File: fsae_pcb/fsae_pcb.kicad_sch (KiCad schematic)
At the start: 0 parts

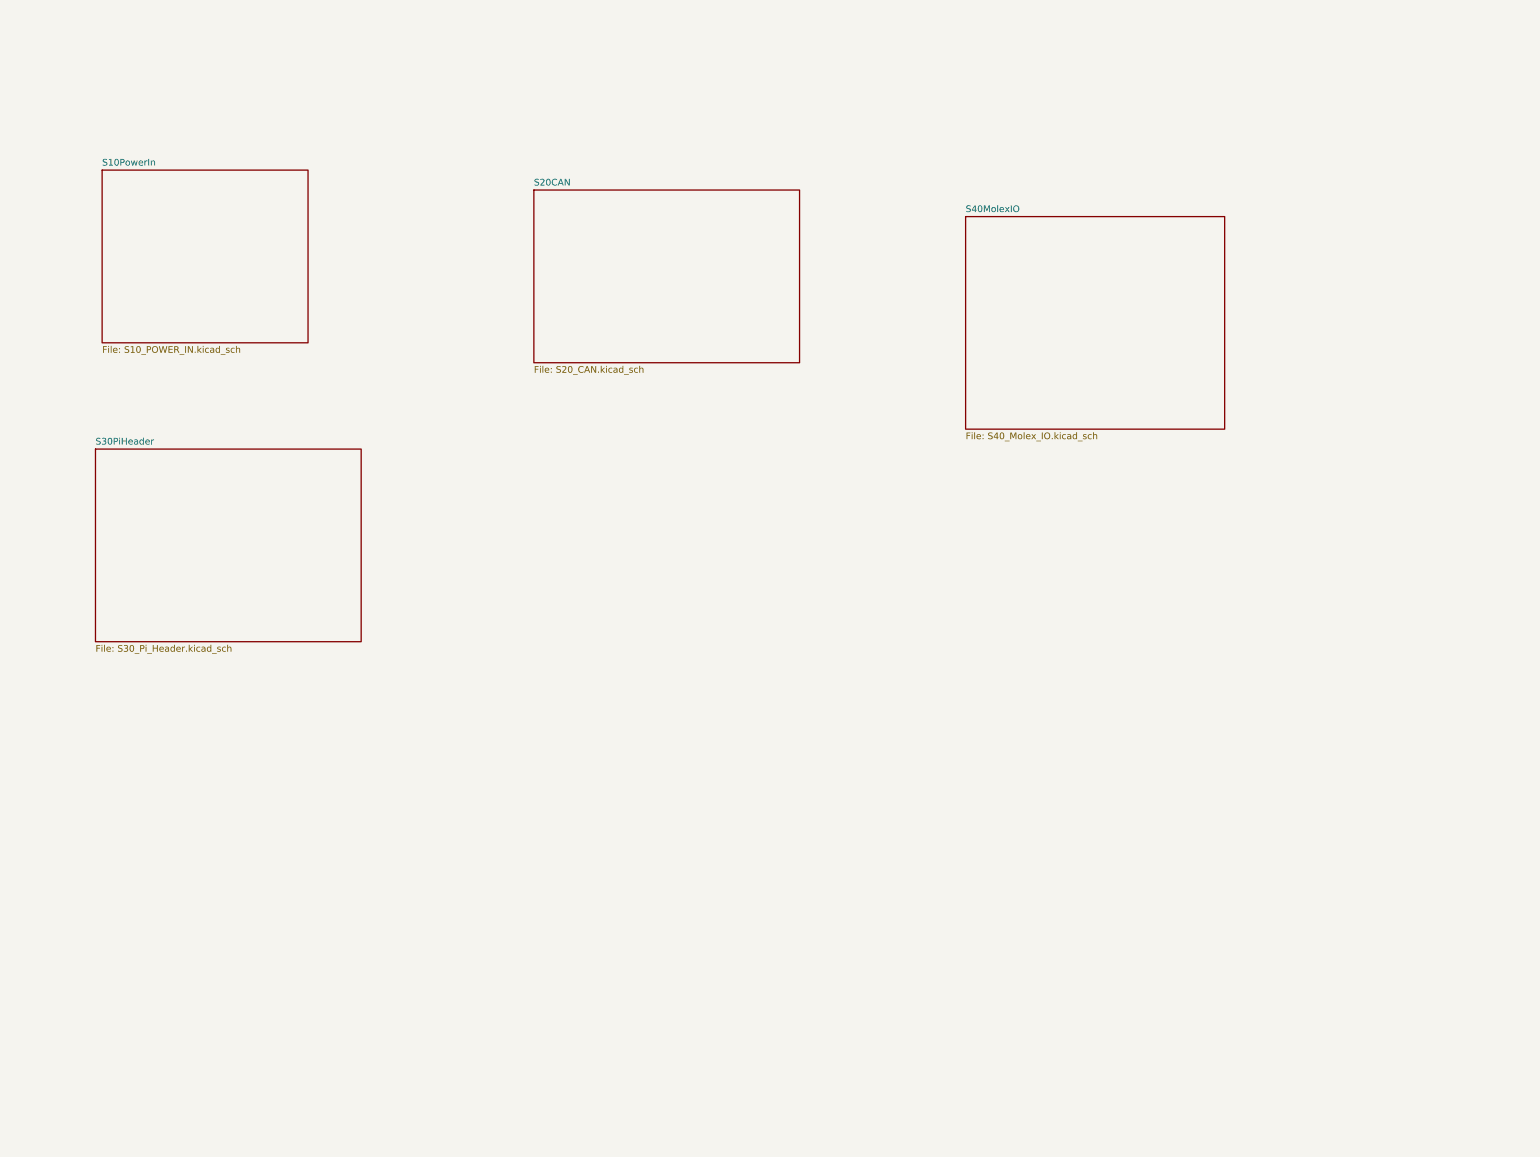
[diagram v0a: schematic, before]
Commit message: new main pcb design
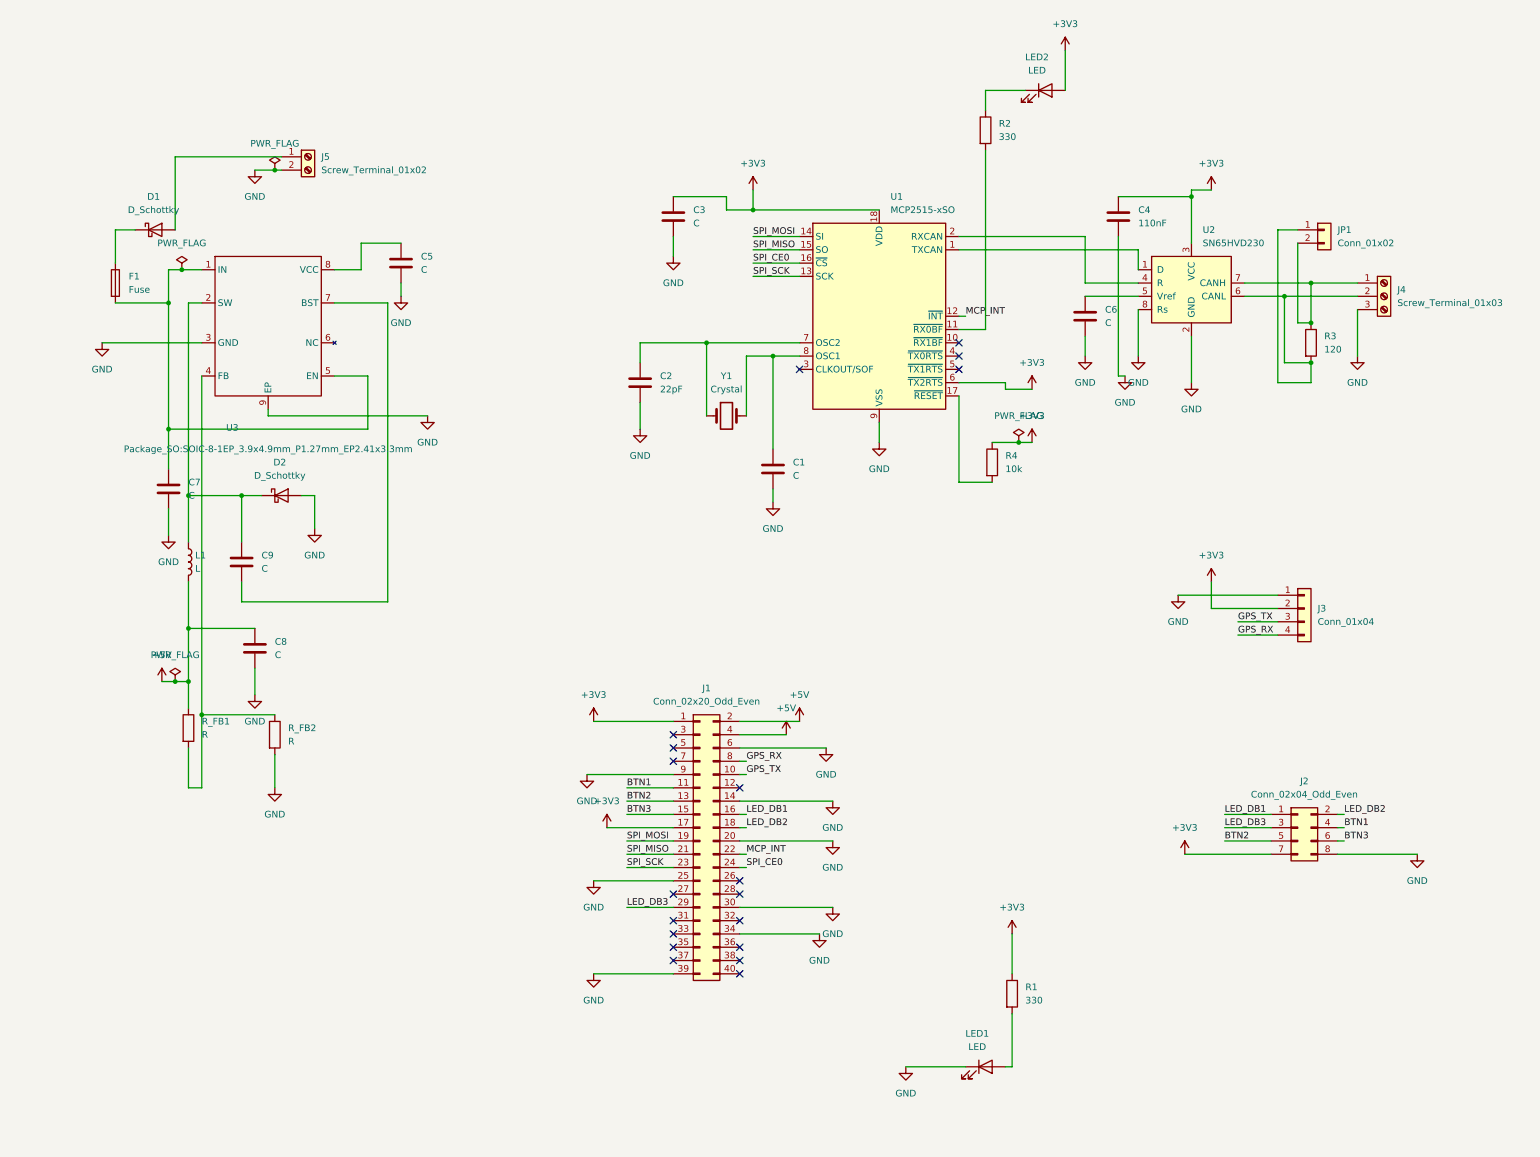
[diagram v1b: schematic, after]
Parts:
- added C1, C3, C5, C6, C7, C8, C9: C, symbol Device:C
- added C2: 22pF, symbol Device:C
- added C4: 110nF, symbol Device:C
- added D1, D2: D_Schottky, symbol Device:D_Schottky
- added F1: Fuse, symbol Device:Fuse
- added J1: Conn_02x20_Odd_Even, symbol Connector_Generic:Conn_02x20_Odd_Even
- added J2: Conn_02x04_Odd_Even, symbol Connector_Generic:Conn_02x04_Odd_Even
- added J3: Conn_01x04, symbol Connector_Generic:Conn_01x04
- added J4: Screw_Terminal_01x03, symbol Connector:Screw_Terminal_01x03
- added J5: Screw_Terminal_01x02, symbol Connector:Screw_Terminal_01x02
- added JP1: Conn_01x02, symbol Connector_Generic:Conn_01x02
- added L1: L, symbol Device:L
- added LED1, LED2: LED, symbol Device:LED
- added R1, R2: 330, symbol Device:R
- added R3: 120, symbol Device:R
- added R4: 10k, symbol Device:R
- added R_FB1, R_FB2: R, symbol Device:R
- added U1: MCP2515-xSO, Package_SO:SOIC-18W_7.5x11.6mm_P1.27mm, symbol Interface_CAN_LIN:MCP2515-xSO
- added U2: SN65HVD230, Package_SO:SOIC-8_3.9x4.9mm_P1.27mm, symbol Interface_CAN_LIN:SN65HVD230
- added U3: ~, Package_SO:SOIC-8-1EP_3.9x4.9mm_P1.27mm_EP2.41x3.3mm, symbol MP1584EN:MP_1
- added Y1: Crystal, symbol Device:Crystal
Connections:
- new net: C9.1, D2.1 (K), L1.1, U3.2 (SW)
- new net: C9.2, U3.7 (BST)
- new net: J4.2 (Pin_2), JP1.1 (Pin_1), R3.2, U2.6 (CANL)
- new net: J4.1 (Pin_1), JP1.2 (Pin_2), R3.1, U2.7 (CANH)
- new net: C2.1, U1.7 (OSC2), Y1.1
- new net: C1.1, U1.8 (OSC1), Y1.2
- new net: R_FB1.2, R_FB2.1, U3.4 (FB)
- new net: C5.1, U3.8 (VCC)
- new net: D1.1 (K), F1.1
- new net: D1.2 (A), J5.1 (Pin_1)
- new net: LED1.2 (A), R1.2
- new net: LED2.1 (K), R2.1
- new net: R2.2, U1.11 (~{RX0BF})
- new net: U1.1 (TXCAN), U2.1 (D)
- new net: U1.2 (RXCAN), U2.4 (R)
- new net: C6.1, U2.5 (Vref)
- new net: C7.1, F1.2, U3.1 (IN), U3.5 (EN)
- new net: R4.2, U1.17 (~{RESET})
- new net +3V3: C3.1, C4.1, J1.1 (Pin_1), J1.17 (Pin_17), J2.7 (Pin_7), J3.2 (Pin_2), LED2.2 (A), R1.1, R4.1, U1.18 (VDD), U1.6 (~{TX2RTS}), U2.3 (VCC)
- new net +5V: C8.1, J1.2 (Pin_2), J1.4 (Pin_4), L1.2, R_FB1.1
- new net BTN1: J1.11 (Pin_11), J2.4 (Pin_4)
- new net BTN2: J1.13 (Pin_13), J2.5 (Pin_5)
- new net BTN3: J1.15 (Pin_15), J2.6 (Pin_6)
- new net GND: C1.2, C2.2, C3.2, C4.2, C5.2, C6.2, C7.2, C8.2, D2.2 (A), J1.14 (Pin_14), J1.20 (Pin_20), J1.25 (Pin_25), J1.30 (Pin_30), J1.34 (Pin_34), J1.39 (Pin_39), J1.6 (Pin_6), J1.9 (Pin_9), J2.8 (Pin_8), J3.1 (Pin_1), J4.3 (Pin_3), J5.2 (Pin_2), LED1.1 (K), R_FB2.2, U1.9 (VSS), U2.2 (GND), U2.8 (Rs), U3.3 (GND), U3.9 (EP)
- new net GPS_RX: J1.8 (Pin_8), J3.4 (Pin_4)
- new net GPS_TX: J1.10 (Pin_10), J3.3 (Pin_3)
- new net LED_DB1: J1.16 (Pin_16), J2.1 (Pin_1)
- new net LED_DB2: J1.18 (Pin_18), J2.2 (Pin_2)
- new net LED_DB3: J1.29 (Pin_29), J2.3 (Pin_3)
- new net MCP_INT: J1.22 (Pin_22), U1.12 (~{INT})
- new net SPI_CE0: J1.24 (Pin_24), U1.16 (~{CS})
- new net SPI_MISO: J1.21 (Pin_21), U1.15 (SO)
- new net SPI_MOSI: J1.19 (Pin_19), U1.14 (SI)
- new net SPI_SCK: J1.23 (Pin_23), U1.13 (SCK)
- no-connect marks 0 -> 19
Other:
- removed sheet S10PowerIn
- removed sheet S20CAN
- removed sheet S30PiHeader
- removed sheet S40MolexIO

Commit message: finished product
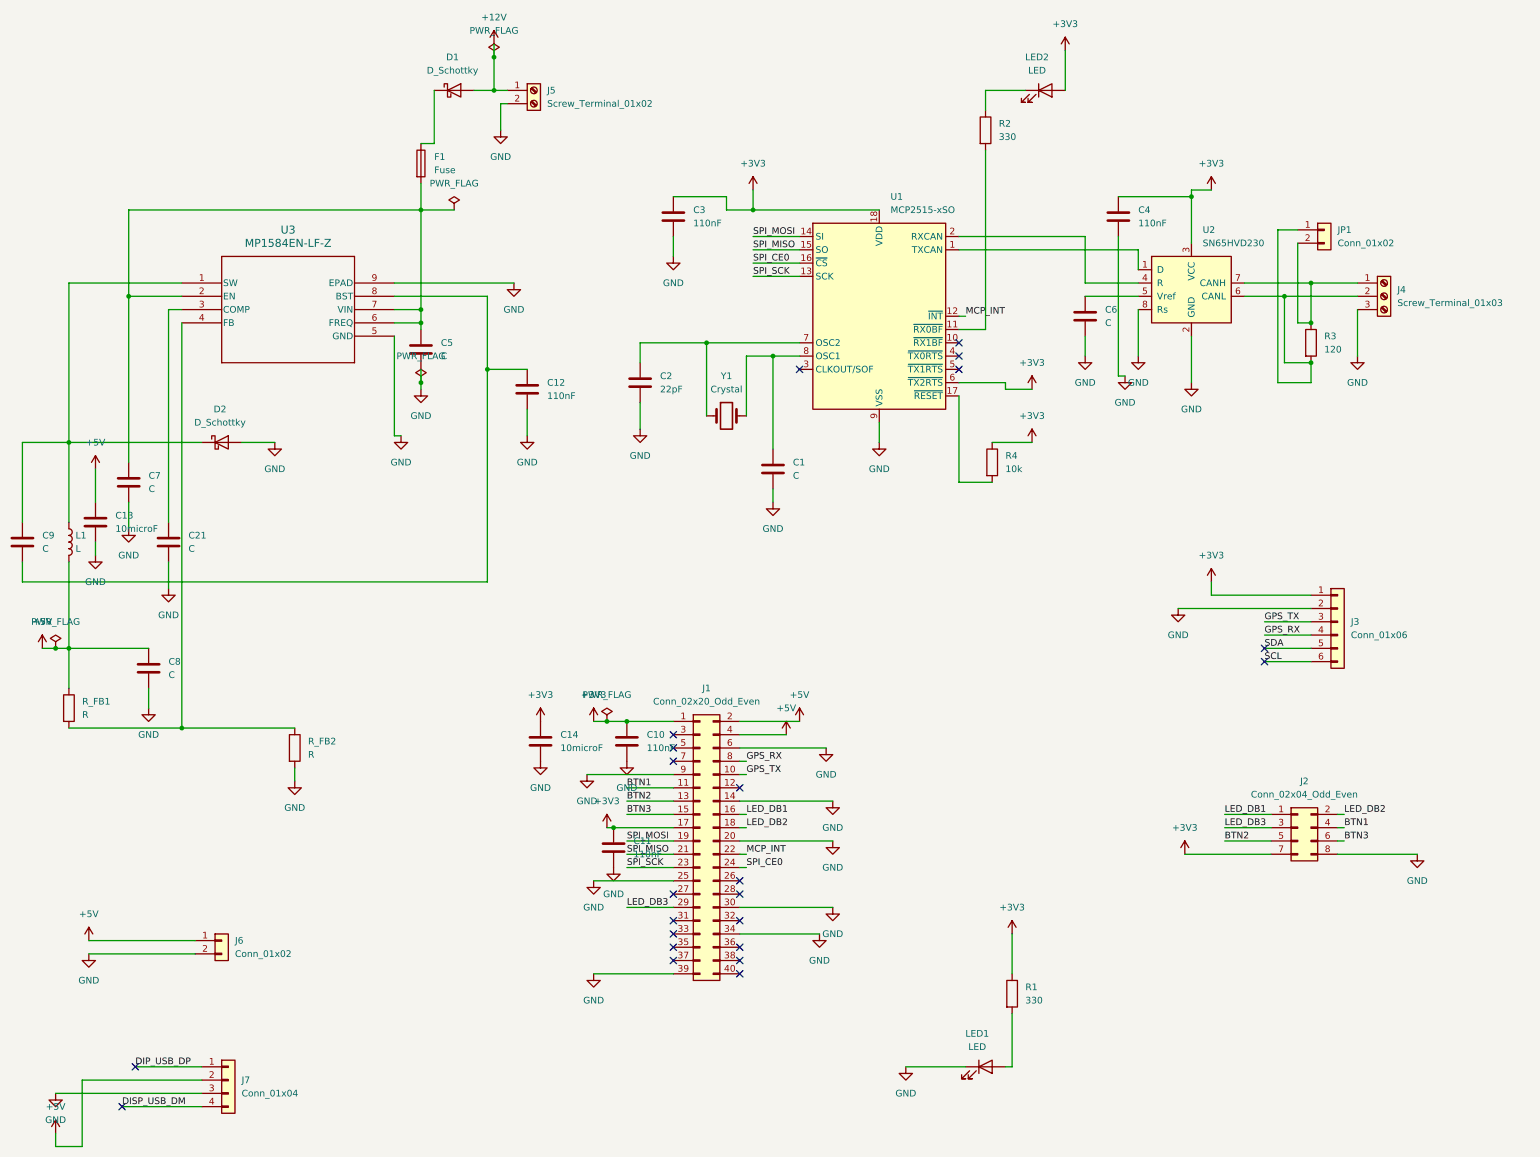
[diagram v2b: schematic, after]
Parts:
- removed J3: Conn_01x04, symbol Connector_Generic:Conn_01x04
- removed U3: ~, Package_SO:SOIC-8-1EP_3.9x4.9mm_P1.27mm_EP2.41x3.3mm, symbol MP1584EN:MP_1
- added C10, C11, C12: 110nF, Capacitor_SMD:C_0805_2012Metric, symbol Device:C
- added C13, C14: 10microF, Capacitor_SMD:C_0805_2012Metric, symbol Device:C
- added C21: C, Capacitor_SMD:C_0805_2012Metric, symbol Device:C
- added J3: Conn_01x06, Connector_PinHeader_2.54mm:PinHeader_1x06_P2.54mm_Vertical, symbol Connector_Generic:Conn_01x06
- added J6: Conn_01x02, Connector_PinHeader_2.54mm:PinHeader_1x02_P2.54mm_Vertical, symbol Connector_Generic:Conn_01x02
- added J7: Conn_01x04, Connector_PinHeader_2.54mm:PinHeader_1x04_P2.54mm_Vertical, symbol Connector_Generic:Conn_01x04
- added U3: MP1584EN-LF-Z, Package_SO:SOIC-8-1EP_3.9x4.9mm_P1.27mm_EP2.29x3mm, symbol 2026-03-05_05-11-51:MP1584EN-LF-Z
- C1, C2, C4, C5, C6, C9: footprint (none) -> Capacitor_SMD:C_0805_2012Metric
- C3: value C -> 110nF; footprint (none) -> Capacitor_SMD:C_0805_2012Metric
- C7, C8: footprint (none) -> Capacitor_SMD:C_1210_3225Metric
- D1, D2: footprint (none) -> Diode_SMD:D_SMA
- F1: footprint (none) -> Fuse:Fuseholder_Clip-5x20mm_Littelfuse_111_Inline_P20.00x5.00mm_D1.05mm_Horizontal
- J1: footprint (none) -> RPi_Hat.pretty-master:Pin_Header_Straight_2x20
- J2: footprint (none) -> Connector_Molex:Molex_Micro-Fit_3.0_43045-0812_2x04_P3.00mm_Vertical
- J4: footprint (none) -> TerminalBlock_Phoenix:TerminalBlock_Phoenix_MKDS-1,5-3-5.08_1x03_P5.08mm_Horizontal
- J5: footprint (none) -> TerminalBlock_Phoenix:TerminalBlock_Phoenix_MKDS-1,5-2-5.08_1x02_P5.08mm_Horizontal
- JP1: footprint (none) -> Connector_PinHeader_2.54mm:PinHeader_1x02_P2.54mm_Vertical
- L1: footprint (none) -> Inductor_SMD:L_Bourns_SRR1260
- LED1, LED2: footprint (none) -> LED_THT:LED_D3.0mm
- R1, R2, R3, R4, R_FB1, R_FB2: footprint (none) -> Resistor_SMD:R_0805_2012Metric
- Y1: footprint (none) -> Crystal:Crystal_HC49-4H_Vertical
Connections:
- net +3V3: now also C10.1, C11.1, C14.1, J3.1 (Pin_1)
- net +5V: now also C13.1, J6.1 (Pin_1), J7.2 (Pin_2)
- net GND: now also C10.2, C11.2, C12.2, C13.2, C14.2, C21.2, J3.2 (Pin_2), J6.2 (Pin_2), J7.3 (Pin_3), U3.5 (GND), U3.9 (EPAD)
- net GPS_RX: now also J3.4 (Pin_4)
- net GPS_TX: now also J3.3 (Pin_3)
- net at C9.1, D2.1 (K), L1.1: now also U3.1 (SW)
- net at C9.2: now also C12.1, U3.8 (BST)
- net at R_FB1.2, R_FB2.1: now also U3.4 (FB)
- net at C5.1: now also C7.1, F1.2, U3.2 (EN), U3.6 (FREQ), U3.7 (VIN)
- net +12V: now reaches D1.2 (A), J5.1 (Pin_1)
- new net: C21.1, U3.3 (COMP)
- new net DIP_USB_DP: J7.1 (Pin_1)
- new net DISP_USB_DM: J7.4 (Pin_4)
- new net SCL: J3.6 (Pin_6)
- new net SDA: J3.5 (Pin_5)
- no-connect marks 19 -> 23
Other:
- moved on the sheet: C5, C7, C8, C9, D1, D2, F1, J5, L1, R_FB1, R_FB2
